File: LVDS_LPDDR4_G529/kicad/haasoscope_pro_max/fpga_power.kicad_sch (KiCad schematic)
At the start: 1 part, among them U3 Ti90G529_Functions

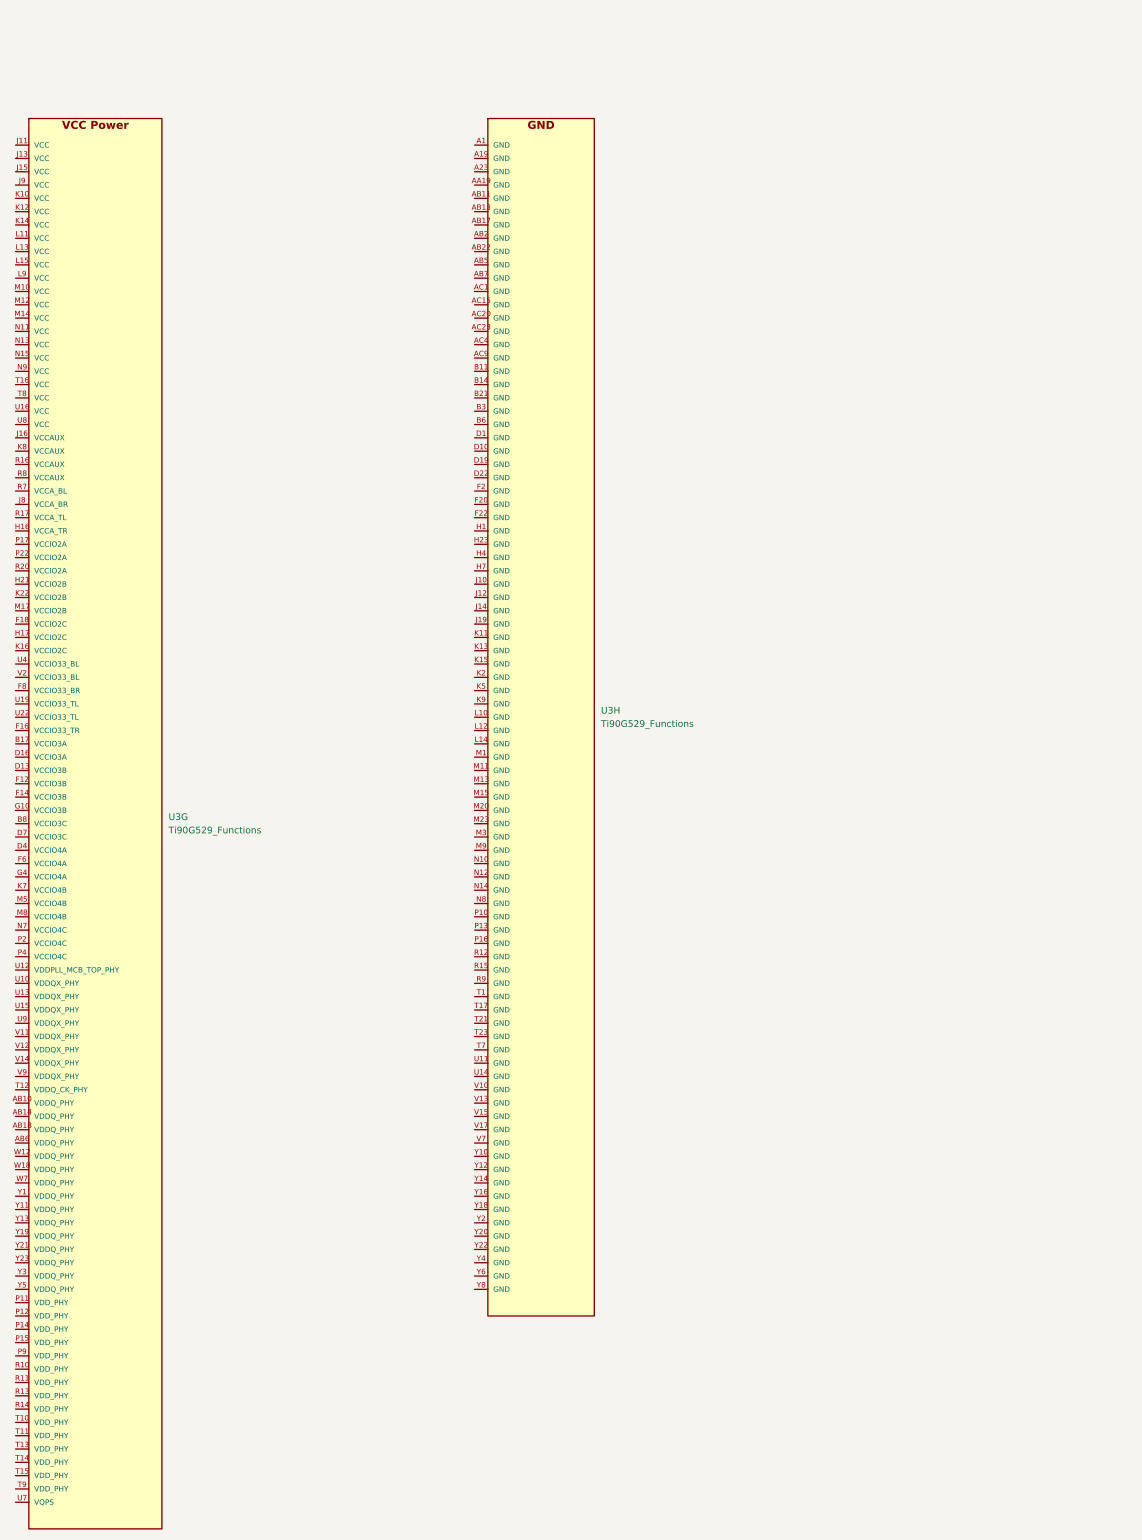
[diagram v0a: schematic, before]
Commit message: Aligned schematics, sort of
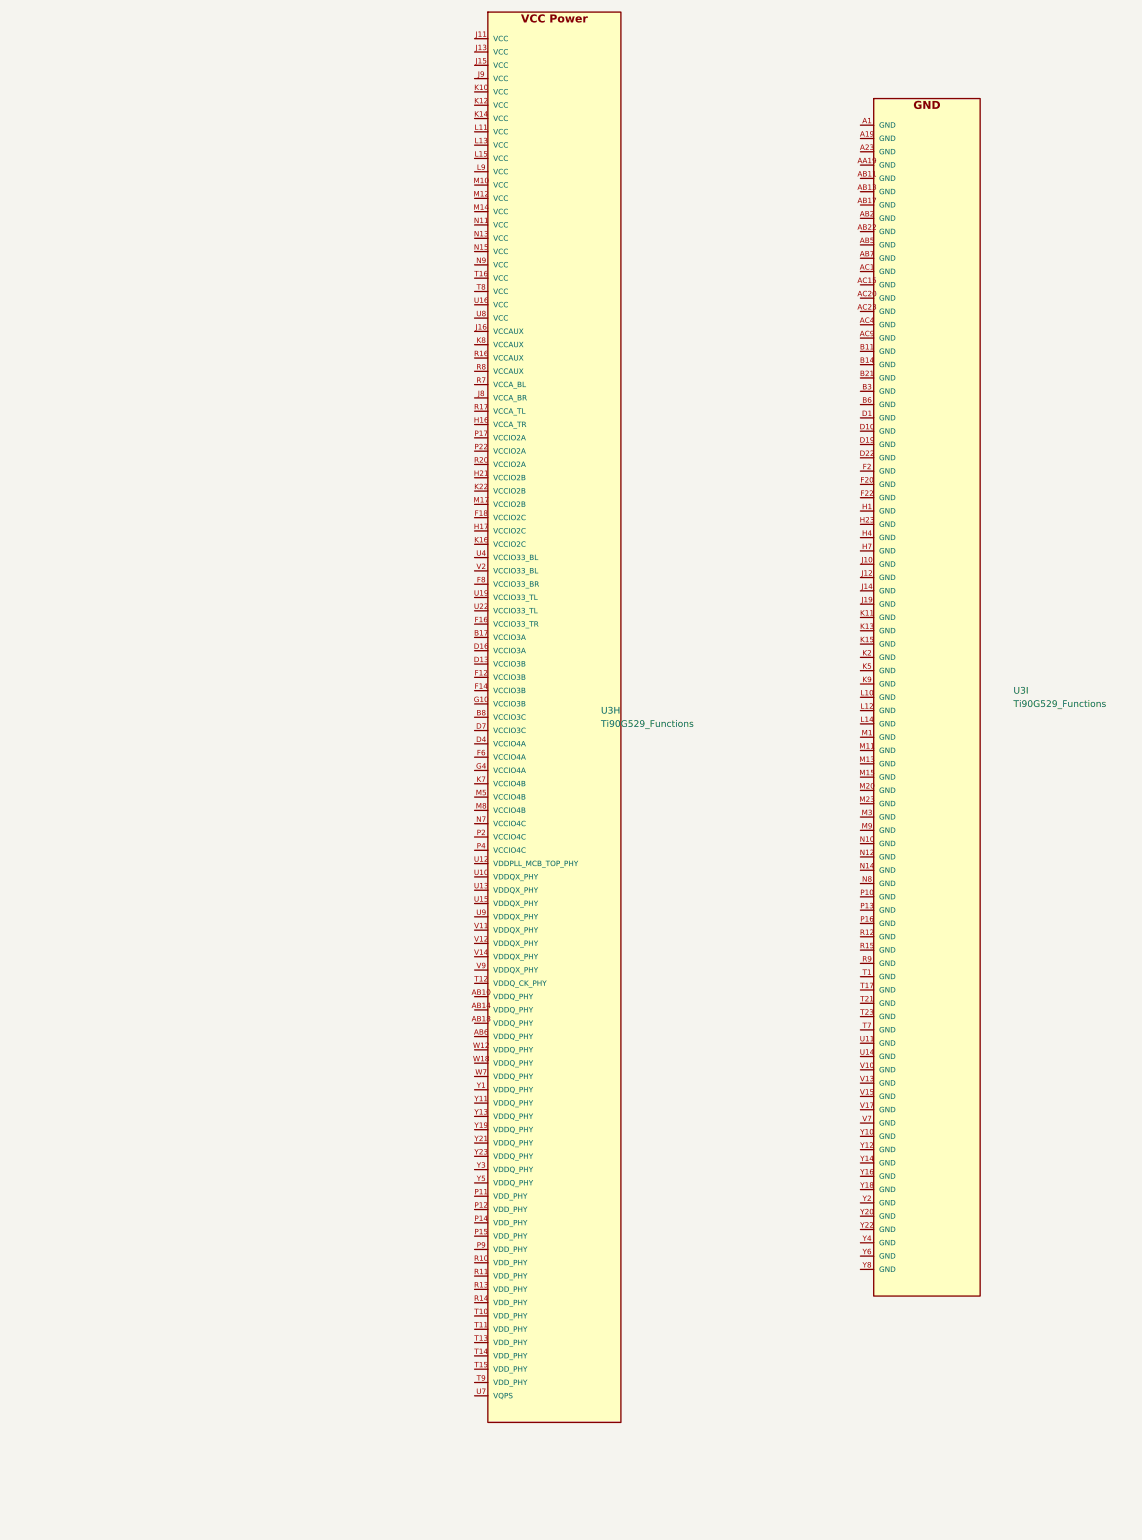
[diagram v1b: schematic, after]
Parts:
- removed unit 7 of U3
- added unit 9 of U3
- U3: footprint G529:BGA-529_23x23_19.0x19.0mm -> haasoscope_pro_adc_fpga_board:BGA-529_23x23_19.0x19.0mm
